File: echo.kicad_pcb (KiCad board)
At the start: 2 copper layers, 99 x 45.5 mm, 82 parts, among them J2 USB4215-03-A, J3 MDC-036, J4 D-SUB 15 Female, J5 0475710001, J6 104031-0811, J7 PJ-320D, J8 RP2040-Zero, J9 SS-52100-004, Q1 BSS138, Q2 BSS138, U1 SN74CBT3257CDR, U2 CH340G, U3 NCP1117 3.3, U4 USBLC6-2SC6, U5 ESP32-WROOM-32, U6 ESP-PSRAM32, X1 12 Mhz

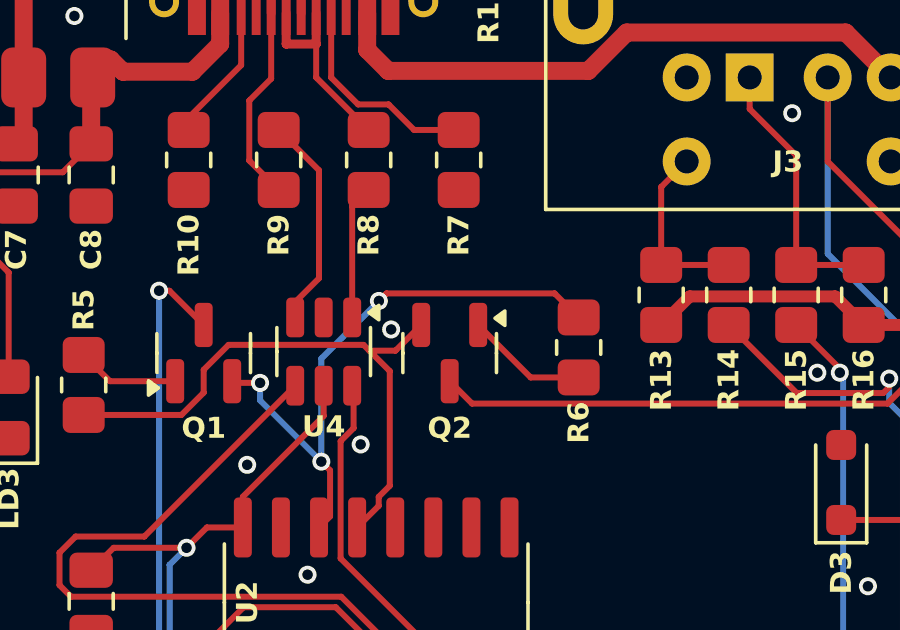
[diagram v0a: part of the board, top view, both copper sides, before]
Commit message: Minor updates
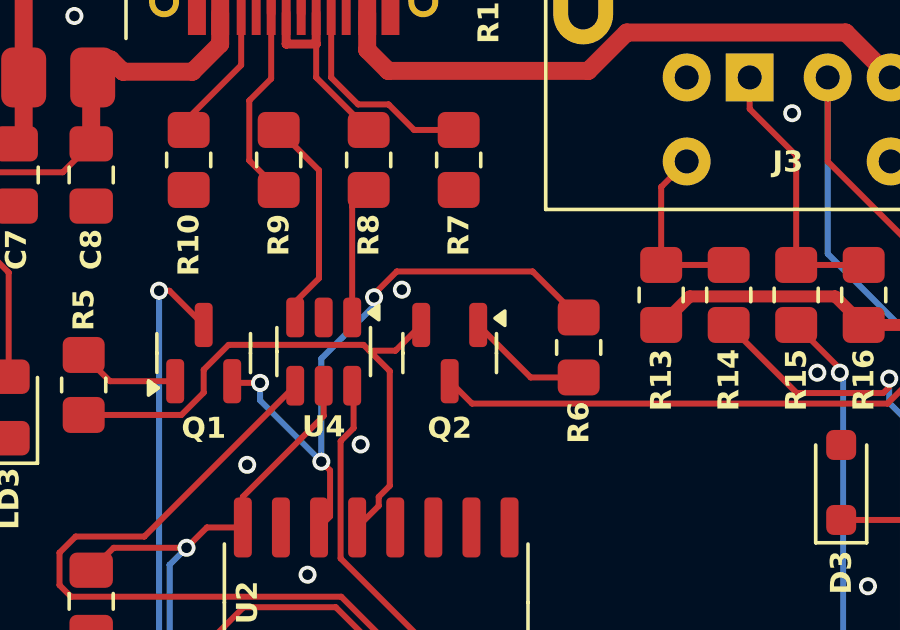
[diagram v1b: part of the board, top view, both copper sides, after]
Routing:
- net Net-(Q1-E): track 20.1 -> 21.0 mm
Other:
- board text added: "Echo"
- board text added: "HW ${VERSION}"
- board text added: "rh1.tech"

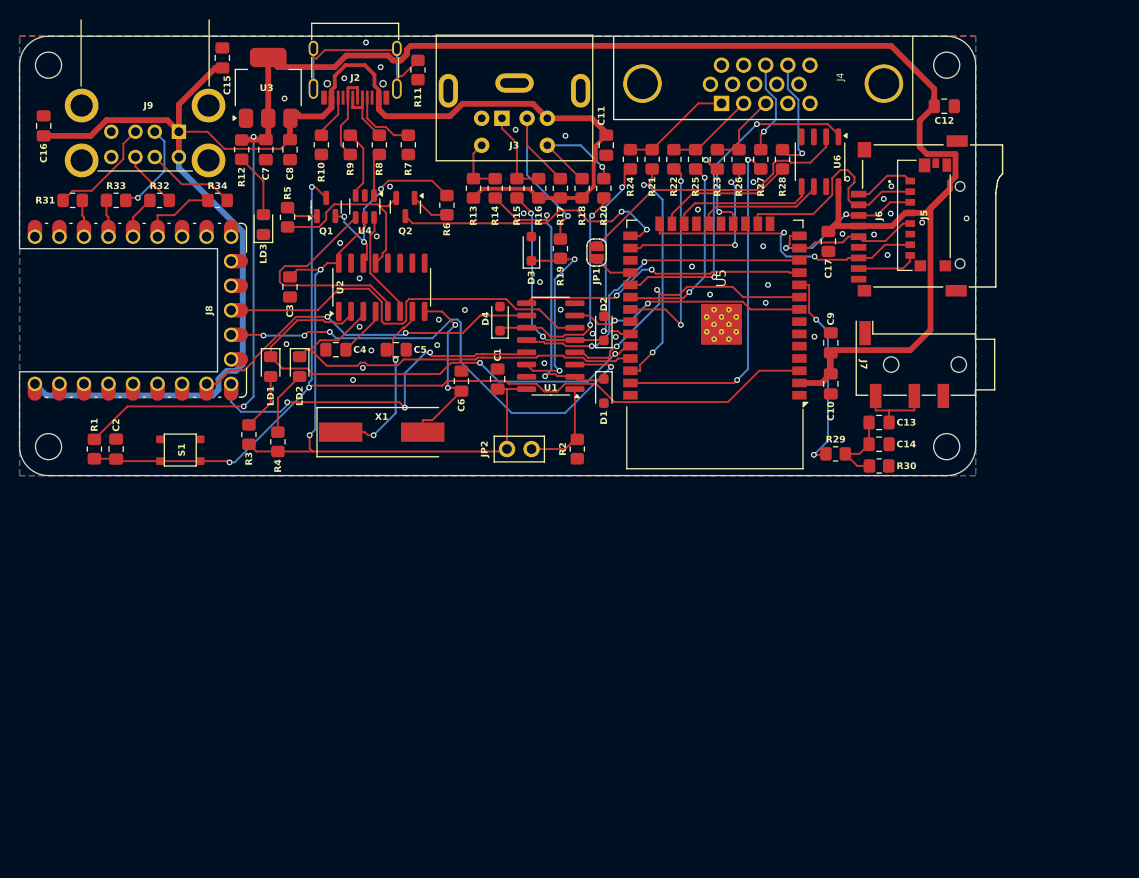
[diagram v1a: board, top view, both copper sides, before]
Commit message: 1.01 WIP
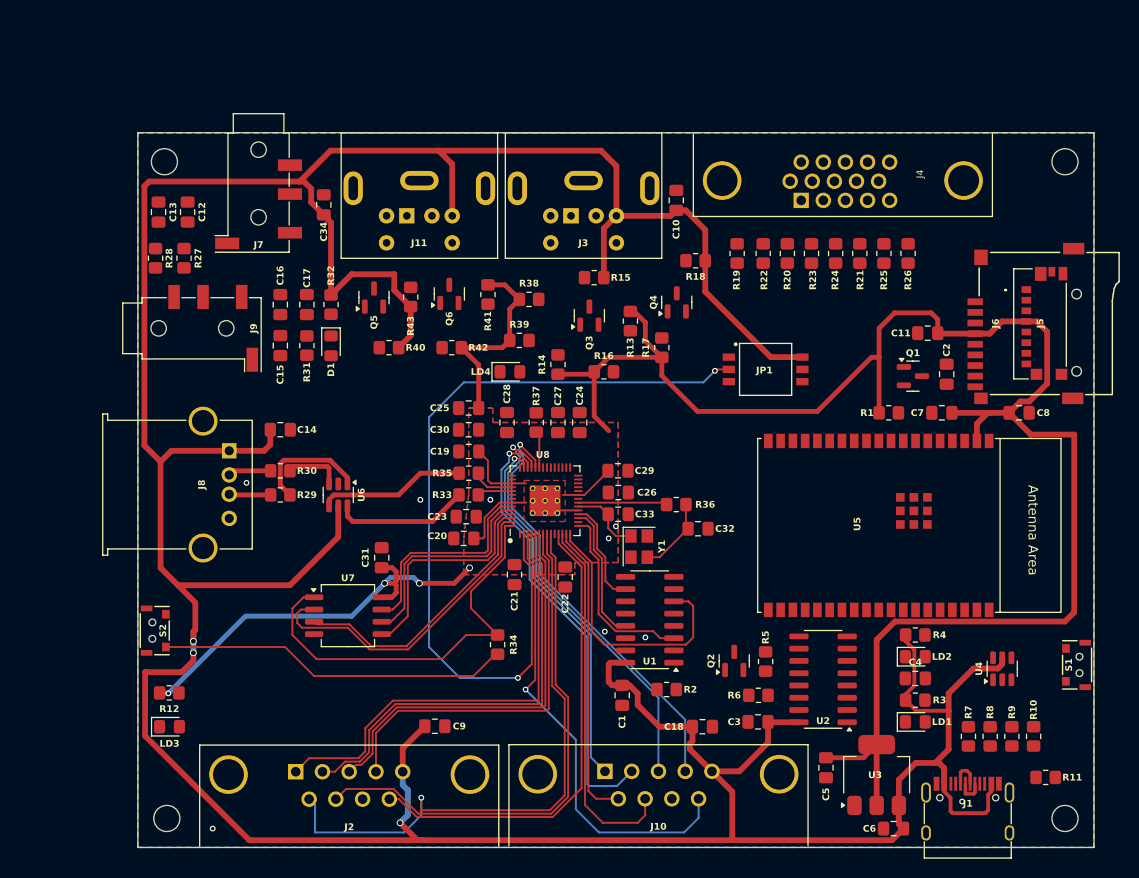
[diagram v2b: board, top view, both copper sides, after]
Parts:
- removed D2, D3, D4: 3V3, FRANK:Diode (SOD-323)
- removed JP2: Input Control, FRANK:Pin Header (1x02)
- removed X1: 12 Mhz, FRANK:Crystal (HC49-S)
- added C18: 100n, FRANK:Capacitor (0805), F.Cu at (209.7, 124.2)
- added C19: 100n, FRANK:Capacitor (0805), F.Cu at (185.5, 95.8)
- added C20: 100n, FRANK:Capacitor (0805), F.Cu at (185.0, 104.8)
- added C21: 100n, FRANK:Capacitor (0805), F.Cu at (190.2, 108.5)
- added C22: 100n, FRANK:Capacitor (0805), F.Cu at (195.5, 108.8)
- added C23: 100n, FRANK:Capacitor (0805), F.Cu at (185.2, 102.5)
- added C24: 100n, FRANK:Capacitor (0805), F.Cu at (197.0, 92.8)
- added C25: 100n, FRANK:Capacitor (0805), F.Cu at (185.5, 91.2)
- added C26: 100n, FRANK:Capacitor (0805), F.Cu at (201.0, 100.0)
- added C27: 100n, FRANK:Capacitor (0805), F.Cu at (194.8, 92.8)
- added C28: 100n, FRANK:Capacitor (0805), F.Cu at (189.5, 92.8)
- added C29: 1u, FRANK:Capacitor (0805), F.Cu at (201.0, 97.8)
- added C30: 1u, FRANK:Capacitor (0805), F.Cu at (185.5, 93.5)
- added C31: 100n, FRANK:Capacitor (0805), F.Cu at (176.5, 106.8)
- added C32: 15p, FRANK:Capacitor (0805), F.Cu at (209.2, 103.8)
- added C33: 15p, FRANK:Capacitor (0805), F.Cu at (201.0, 102.2)
- added C34: 100n, FRANK:Capacitor (0805), F.Cu at (170.5, 70.2)
- added J1: USB4215-03-A, FRANK:USB Type C, F.Cu at (237.2, 137.8)
- added J10: D-SUB 9 Male, FRANK:D-SUB (9 pin, male, top mount), F.Cu at (199.6, 128.9)
- added J11: MDC-036, FRANK:MiniDIN (6 Pin, female), F.Cu at (179.1, 71.3)
- added LD4: Blue, FRANK:LED (0805), F.Cu at (189.8, 87.5)
- added Q3: AO3400A, FRANK:SOT-23, F.Cu at (198.0, 81.7)
- added Q4: AO3400A, FRANK:SOT-23, F.Cu at (207.1, 80.3)
- added Q5: AO3400A, FRANK:SOT-23, F.Cu at (175.7, 79.8)
- added Q6: AO3400A, FRANK:SOT-23, F.Cu at (183.5, 79.4)
- added R35: 27R, FRANK:Resistor (0805), F.Cu at (185.5, 98.0)
- added R36: 1K, FRANK:Resistor (0805), F.Cu at (207.0, 101.2)
- added R37: 1K, FRANK:Resistor (0805), F.Cu at (192.5, 92.8)
- added R38: 22K, FRANK:Resistor (0805), F.Cu at (191.8, 80.0)
- added R39: 4.7K, FRANK:Resistor (0805), F.Cu at (190.8, 84.2)
- added R40: 22K, FRANK:Resistor (0805), F.Cu at (177.2, 85.0)
- added R41: 22K, FRANK:Resistor (0805), F.Cu at (187.5, 79.5)
- added R42: 4.7K, FRANK:Resistor (0805), F.Cu at (183.8, 85.0)
- added R43: 22K, FRANK:Resistor (0805), F.Cu at (179.5, 79.8)
- added S2: Boot, FRANK:TACT-SIDE-4623, F.Cu at (152.8, 114.3)
- added U7: W25Q128JVSIQ, FRANK:SOIC-8, F.Cu at (173.0, 112.8)
- added U8: RP2040, FRANK:QFN 56, F.Cu at (193.4, 100.8)
- added Y1: 12 MHz, FRANK:Crystal (3225), F.Cu at (203.2, 105.6)
- C12: value 100n -> 10u
- C13: value 10u -> 33n
- C14: value 33n -> 10u
- C15, C16, C8, C9: value 10u -> 100n
- C5, C6: value 15p -> 10u
- D1: value 3V3 -> Zener 3V3; footprint FRANK:Diode (SOD-323) -> FRANK:Diode (0805)
- J2: value USB4215-03-A -> D-SUB 9 Male; footprint FRANK:USB Type C -> FRANK:D-SUB (9 pin, male, top mount)
- J8: value RP2040-Zero -> 676430910; footprint FRANK:Raspberry Pi Zero -> FRANK:USB Type A (single)
- J9: value SS-52100-004 -> PJ-320D; footprint FRANK:USB Type A (stacked) -> FRANK:Jack (3.5mm, PJ-320D)
- JP1: value Jumper (Solder) -> Main Jumpers; footprint FRANK:Jumper (solder) -> FRANK:SW_DS05-127-2-03BK-SMT-TR
- R13, R16, R18: value 1K -> 22K
- R14: value 100R -> 4.7K
- R15: value 100R -> 22K
- R17: value 1K -> 4.7K
- R19, R20: value 100R -> 330R
- R22, R23: value 330R -> 1K
- R25, R26: value 1K -> 100R
- R28: value 100R -> 150R
- R29: value 100R -> 22R
- R30: value 150R -> 22R
- R31, R32: value 22R -> 10K
- R33: value 22R -> 27R
- R34: value 22R -> 1K
- S1: footprint FRANK:Button (SMD, 3x3mm, 1-1) -> FRANK:TACT-SIDE-4623
- U2: value CH340G -> CH340C
- U5: value ESP32-WROOM-32 -> ESP32-WROVER-E; footprint RF_Module:ESP32-WROOM-32 -> FRANK:ESP32-WROVER-E
- U6: value ESP-PSRAM32 -> USBLC6-2SC6; footprint FRANK:SO-8 -> FRANK:SOT-23-6
- moved R11 97.9 mm to (245.2, 129.5), turned to 0 degrees
- moved S1 97.7 mm to (248.8, 117.8), turned to -90 degrees
- moved R10 95.9 mm to (244.0, 125.2), turned to -90 degrees
- moved U3 95.0 mm to (227.8, 129.2)
- moved R9 91.9 mm to (241.8, 125.2)
- moved R8 88.0 mm to (239.5, 125.2), turned to -90 degrees
- moved C2 86.3 mm to (235.0, 87.8)
- moved R7 84.4 mm to (237.2, 125.2), turned to -90 degrees
- moved R1 82.3 mm to (229.0, 91.8), turned to 180 degrees
- moved U4 81.5 mm to (240.8, 118.2), turned to 90 degrees
- moved C8 80.3 mm to (242.5, 91.8), turned to 0 degrees
- moved C12 79.1 mm to (156.4, 71.0), turned to -90 degrees
- moved J2 77.7 mm to (167.6, 128.9), turned to 0 degrees
- moved C13 77.7 mm to (153.4, 71.0), turned to -90 degrees
- moved LD1 76.2 mm to (231.8, 123.8), turned to 0 degrees
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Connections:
- net /ESP32/IO35 renamed /ESP_IO35
- net /ESP32/SENSOR_VN renamed /SENSOR_VN
- net /ESP32/SENSOR_VP renamed /SENSOR_VP
- net /SD Card/DAT1 renamed /DAT1
- net /SD Card/DAT2 renamed /DAT2
- net /SD Card/DET renamed /DET
- net /SD Card/POL renamed /POL
- C1 pad 2: VCC -> VBUS
- C10 pad 1: +3V3 -> VBUS
- C11 pad 1: VBUS -> GND
- C11 pad 2: GND -> +3V3
- C12 pad 1: GND -> /Audio Out/A_OUT
- C12 pad 2: +3V3 -> Net-(C12-Pad2)
- C13 pad 1: /Audio Out/A_OUT -> GND
- C13 pad 2: Net-(C13-Pad2) -> Net-(C12-Pad2)
- C14 pad 2: Net-(C13-Pad2) -> VBUS
- C15 pad 1: VBUS -> GND
- C15 pad 2: GND -> /Tape In/G
- C16 pad 1: VBUS -> /LOAD_IN
- C16 pad 2: GND -> /Tape In/L
- C17 pad 1: +3V3 -> /LOAD_IN
- C17 pad 2: GND -> /Tape In/R
- C3 pad 1: VCC -> VBUS
- C5 pad 1: Net-(U2-XI) -> +3V3
- C6 pad 1: Net-(U2-XO) -> VBUS
- C8 pad 1: VBUS -> +3V3
- C9 pad 1: +3V3 -> VBUS
- D1 pad 1: /KB_CLK_3V -> /LOAD_IN
- J2 pad 1: GND -> /GPIO2
- J2 pad 2: VBUS -> /GPIO3
- J2 pad 3: unconnected-(J2-SBU2-Pad3) -> /GPIO4
- J2 pad 4: Net-(J2-CC1) -> /GPIO5
- J2 pad 5: Net-(J2-DN1) -> VBUS
- J2 pad 6: Net-(J2-DP1) -> /GPIO6
- J2 pad 7: Net-(J2-DN1) -> /GPIO7
- J2 pad 8: Net-(J2-DP1) -> GND
- J2 pad 9: unconnected-(J2-SBU1-Pad9) -> /GPIO8
- J3 pad 1: Net-(J3-Pad1) -> /PS2 KB/DATA
- J3 pad 2: Net-(J3-Pad2) -> unconnected-(J3-Pad2)
- J3 pad 5: Net-(J3-Pad5) -> /PS2 KB/CLK
- J3 pad 6: Net-(J3-Pad6) -> unconnected-(J3-Pad6)
- J8 pad 1: /ZGPIO0 -> VBUS
- J8 pad 2: /ZGPIO1 -> Net-(J8-D-)
- J8 pad 3: /ZGPIO2 -> Net-(J8-D+)
- J8 pad 4: /ZGPIO3 -> GND
- J8 pad 5: /ZGPIO4 -> GND
- JP1 pad 1: Net-(JP1-A) -> /SN74_S
- JP1 pad 2: /ESP_IO17 -> /GPIO0
- R10 pad 2: Net-(J2-CC2) -> Net-(J1-CC2)
- R11 pad 1: Net-(J2-SHIELD) -> Net-(J1-SHIELD)
- R13 pad 1: VBUS -> +3V3
- R13 pad 2: Net-(J3-Pad5) -> /KB_CLK_3V
- R14 pad 1: Net-(J3-Pad5) -> +3V3
- R14 pad 2: /KB_CLK_3V -> Net-(Q3-G)
- R15 pad 1: Net-(J3-Pad1) -> VBUS
- R15 pad 2: /KB_DATA_3V -> /PS2 KB/CLK
- R16 pad 1: VBUS -> +3V3
- R16 pad 2: Net-(J3-Pad1) -> /KB_DATA_3V
- R17 pad 1: VBUS -> +3V3
- R17 pad 2: Net-(J3-Pad2) -> Net-(Q4-G)
- R18 pad 2: Net-(J3-Pad6) -> /PS2 KB/DATA
- R19 pad 1: Net-(J3-Pad2) -> /ESP_IO22
- R19 pad 2: /MS_DATA_3V -> Net-(J4-Pad1)
- R20 pad 1: Net-(J3-Pad6) -> /ESP_IO19
- R20 pad 2: /MS_CLK_3V -> Net-(J4-Pad2)
- R21 pad 1: /ESP_IO22 -> /ESP_IO5
- R21 pad 2: Net-(J4-Pad1) -> Net-(J4-Pad3)
- R22 pad 1: /ESP_IO19 -> /ESP_IO21
- R22 pad 2: Net-(J4-Pad2) -> Net-(J4-Pad1)
- R23 pad 1: /ESP_IO5 -> /ESP_IO18
- R23 pad 2: Net-(J4-Pad3) -> Net-(J4-Pad2)
- R24 pad 1: /ESP_IO21 -> /ESP_IO4
- R24 pad 2: Net-(J4-Pad1) -> Net-(J4-Pad3)
- R25 pad 1: /ESP_IO18 -> Net-(J4-Pad13)
- R25 pad 2: Net-(J4-Pad2) -> /ESP_IO23
- R26 pad 1: /ESP_IO4 -> Net-(J4-Pad14)
- R26 pad 2: Net-(J4-Pad3) -> /ESP_IO15
- R27 pad 1: Net-(J4-Pad13) -> /ESP_IO25
- R27 pad 2: /ESP_IO23 -> Net-(C12-Pad2)
- R28 pad 1: Net-(J4-Pad14) -> GND
- R28 pad 2: /ESP_IO15 -> Net-(C12-Pad2)
- R29 pad 1: /ESP_IO25 -> Net-(R29-Pad1)
- R29 pad 2: Net-(C13-Pad2) -> Net-(J8-D+)
- R3 pad 2: VCC -> VBUS
- R30 pad 1: GND -> Net-(R30-Pad1)
- R30 pad 2: Net-(C13-Pad2) -> Net-(J8-D-)
- R31 pad 1: /ZGPIO2 -> /LOAD_IN
- R31 pad 2: Net-(J9-D1+) -> GND
- R32 pad 1: /ZGPIO4 -> /LOAD_IN
- R32 pad 2: Net-(J9-D2+) -> VBUS
- R33 pad 1: /ZGPIO3 -> /RP_D+
- R33 pad 2: Net-(J9-D1-) -> Net-(U8-USB_DP)
- R34 pad 1: /ZGPIO5 -> /RP2040/QSPI_SS
- R34 pad 2: Net-(J9-D2-) -> Net-(R34-Pad2)
- R4 pad 1: VCC -> VBUS
- R7 pad 2: Net-(J2-CC1) -> Net-(J1-CC1)
- R8 pad 2: Net-(J2-DN1) -> Net-(J1-DN1)
- R9 pad 2: Net-(J2-DP1) -> Net-(J1-DP1)
- U1 pad 10: /ZGPIO15 -> /GPIO15
- U1 pad 13: /ZGPIO14 -> /GPIO14
- U1 pad 16: VCC -> VBUS
- U1 pad 3: /ZGPIO12 -> /GPIO12
- U1 pad 6: /ZGPIO11 -> /GPIO11
- U2 pad 16: VCC -> VBUS
- U2 pad 7: Net-(U2-XI) -> unconnected-(U2-XI-Pad7)
- U2 pad 8: Net-(U2-XO) -> unconnected-(U2-XO-Pad8)
- U4 pad 5: VCC -> VBUS
- U5 pad 17: /ESP32/SHD_SD2 -> (no net)
- U5 pad 18: /ESP_SWP_SD3 -> (no net)
- U5 pad 19: /ESP32/SCS_CMD -> (no net)
- U5 pad 20: /ESP_SCK_CLK -> (no net)
- U5 pad 21: /ESP32/SDO_SD0 -> (no net)
- U5 pad 22: /ESP_SDI_SD1 -> (no net)
- U5 pad 27: /ESP32/IO16 -> (no net)
- U5 pad 28: /ESP_IO17 -> (no net)
- U5 pad 32: unconnected-(U5-NC-Pad32) -> (no net)
- U5 pad 6: /ESP32/IO34 -> /ESP_IO34
- U6 pad 1: /ESP_SWP_SD3 -> Net-(R29-Pad1)
- U6 pad 2: Net-(JP1-A) -> GND
- U6 pad 3: unconnected-(U6-SIO2-Pad3) -> Net-(R30-Pad1)
- U6 pad 4: GND -> /RP_D-
- U6 pad 5: /ESP_SDI_SD1 -> VBUS
- U6 pad 6: /ESP_SCK_CLK -> /RP_D+
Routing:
- net VBUS: track 153.8 -> 418.8 mm, vias 0 -> 3
- net /ESP_EN: track 102.4 -> 0.00 mm, vias 3 -> 0
- net /GPIO0: track 0.00 -> 83.3 mm, vias 0 -> 2
- net VCC: track 67.3 -> 0.00 mm, vias 2 -> 0
- net /GPIO6: track 0.00 -> 62.0 mm, vias 0 -> 1
- net /GPIO7: track 0.00 -> 54.2 mm
- net /ZGPIO12: track 53.3 -> 0.00 mm, vias 4 -> 0
- net /ESP_IO3: track 52.1 -> 0.00 mm, vias 2 -> 0
- net /GPIO8: track 0.00 -> 49.2 mm
- net /GPIO1: track 0.00 -> 47.7 mm, vias 0 -> 1
- net /GPIO2: track 0.00 -> 47.2 mm
- net /GPIO28: track 0.00 -> 46.4 mm, vias 0 -> 1
- net /GPIO26: track 0.00 -> 45.0 mm, vias 0 -> 1
- net /GPIO3: track 0.00 -> 44.9 mm
- net /GPIO27: track 0.00 -> 43.9 mm, vias 0 -> 1
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- added copper zone on B.Cu, net +3V3
- added copper zone on F.Cu, net +3V3
- added copper zone on F.Cu, net Net-(U8-VREG_VOUT)
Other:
- board size 99 x 45.5 mm -> 99 x 74 mm
- board text removed: "Echo"
- board text removed: "HW ${VERSION}"
- board text removed: "rh1.tech"
